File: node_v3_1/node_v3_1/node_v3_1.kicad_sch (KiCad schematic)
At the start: 69 parts, among them J1 Conn_Coaxial, J2 12402012E212A, J3 Micro_SD_Card, J4 VIN, J5 BAT, J7 DBG, J8 Conn_01x16_Pin, Q1 2N3904, U1 RST, U2 W25Q128JVS, U3 ADP2108AUJ-3.3, U4 RP2040, U5 RFM69HCW, U6 CAT3200-5, U7 MCP7940N-xSN, U8 MCP73831T-2ACI_OT, U9 BOOTSEL, Y1 445C35A12M00000, Y2 SC32S-7PF20PPM

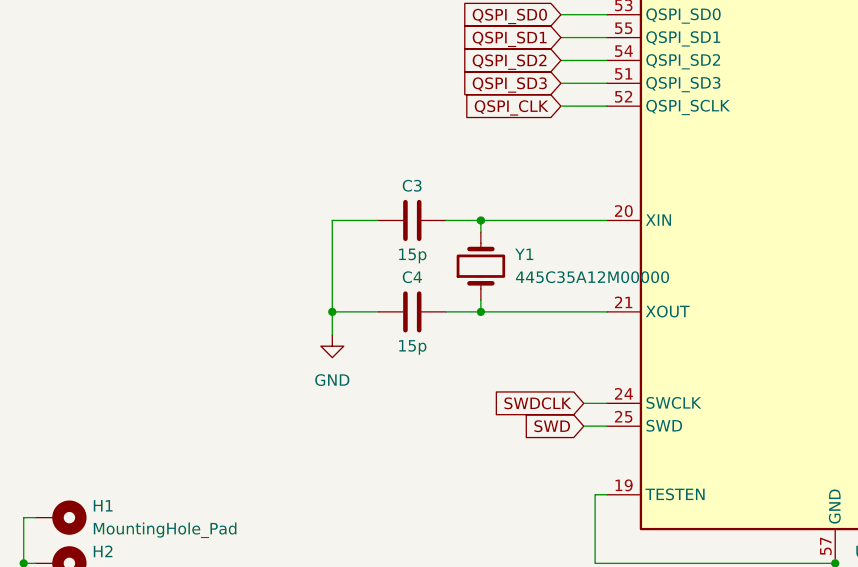
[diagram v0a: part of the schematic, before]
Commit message: updates
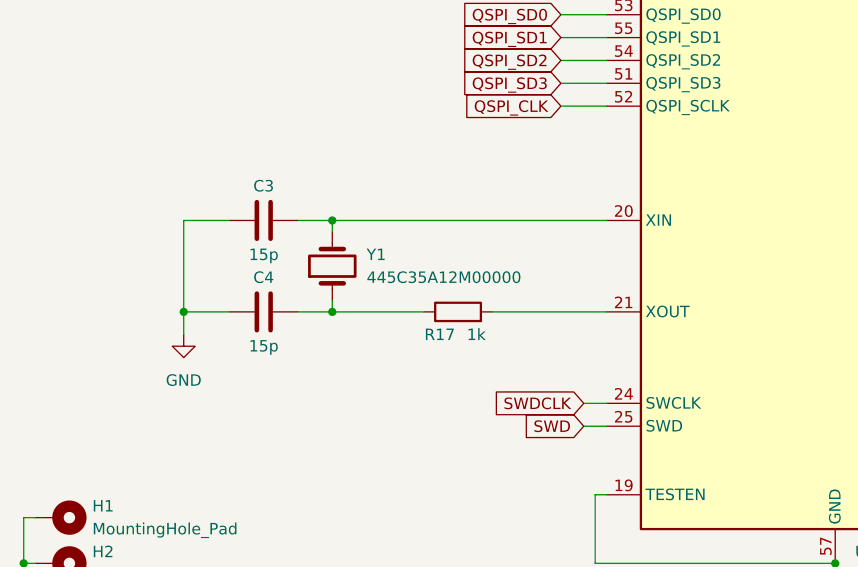
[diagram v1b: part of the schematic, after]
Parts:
- added R17: 1k, symbol Device:R
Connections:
- net at C4.2, Y1.1: now also R17.1; no longer U4.21 (XOUT)
- new net: R17.2, U4.21 (XOUT)
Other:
- moved on the sheet: C3, C4, Y1
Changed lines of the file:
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@@
 	)
 	(junction
-		(at 55.88 241.3)
+		(at 39.37 241.3)
 		(diameter 0)
 		(color 0 0 0 0)
@@
 	)
 	(junction
-		(at 72.39 241.3)
+		(at 55.88 231.14)
 		(diameter 0)
 		(color 0 0 0 0)
 	)
 	(junction
-		(at 72.39 231.14)
+		(at 250.19 248.92)
 		(diameter 0)
 		(color 0 0 0 0)
 	)
 	(junction
-		(at 250.19 248.92)
+		(at 46.99 123.19)
 		(diameter 0)
 		(color 0 0 0 0)
 	)
 	(junction
-		(at 46.99 123.19)
+		(at 21.59 279.4)
 		(diameter 0)
 		(color 0 0 0 0)
 	)
 	(junction
-		(at 21.59 279.4)
+		(at 55.88 241.3)
 		(diameter 0)
 		(color 0 0 0 0)
@@
 	(wire
 		(pts
-			(xy 72.39 240.03) (xy 72.39 241.3)
+			(xy 55.88 240.03) (xy 55.88 241.3)
 		)
 		(stroke
@@
 	(wire
 		(pts
-			(xy 72.39 232.41) (xy 72.39 231.14)
+			(xy 55.88 232.41) (xy 55.88 231.14)
 		)
 		(stroke
@@
 	(wire
 		(pts
-			(xy 72.39 231.14) (xy 86.36 231.14)
+			(xy 55.88 231.14) (xy 86.36 231.14)
 		)
 		(stroke
@@
 	(wire
 		(pts
+			(xy 73.66 241.3) (xy 86.36 241.3)
+		)
+		(stroke
+			(width 0)
+			(type default)
+		)
+	)
+	(wire
+		(pts
 			(xy 36.83 101.6) (xy 40.64 101.6)
 		)
@@
 	(wire
 		(pts
-			(xy 55.88 231.14) (xy 55.88 241.3)
+			(xy 39.37 231.14) (xy 39.37 241.3)
 		)
 		(stroke
@@
 	(wire
 		(pts
+			(xy 55.88 241.3) (xy 66.04 241.3)
+		)
+		(stroke
+			(width 0)
+			(type default)
+		)
+	)
+	(wire
+		(pts
 			(xy 246.38 226.06) (xy 246.38 229.87)
 		)
@@
 	(wire
 		(pts
-			(xy 60.96 231.14) (xy 55.88 231.14)
+			(xy 44.45 231.14) (xy 39.37 231.14)
 		)
 		(stroke
@@
 	(wire
 		(pts
-			(xy 55.88 241.3) (xy 60.96 241.3)
+			(xy 39.37 241.3) (xy 44.45 241.3)
 		)
 		(stroke
@@
 	(wire
 		(pts
-			(xy 55.88 241.3) (xy 55.88 243.84)
+			(xy 39.37 241.3) (xy 39.37 243.84)
 		)
 		(stroke
@@
 	(wire
 		(pts
-			(xy 72.39 241.3) (xy 86.36 241.3)
-		)
-		(stroke
-			(width 0)
-			(type default)
-		)
-	)
-	(wire
-		(pts
 			(xy 137.16 198.12) (xy 139.7 198.12)
 		)
@@
 	(wire
 		(pts
-			(xy 72.39 241.3) (xy 68.58 241.3)
+			(xy 55.88 241.3) (xy 52.07 241.3)
 		)
 		(stroke
@@
 	(wire
 		(pts
-			(xy 72.39 231.14) (xy 68.58 231.14)
+			(xy 55.88 231.14) (xy 52.07 231.14)
 		)
 		(stroke
@@
 	(symbol
 		(lib_id "Device:Crystal")
-		(at 72.39 236.22 90)
+		(at 55.88 236.22 90)
 		(unit 1)
 		(exclude_from_sim no)
@@
 		(on_board yes)
 		(dnp no)
-		(fields_autoplaced yes)
 		(property "Reference" "Y1"
-			(at 76.2 234.95 90)
+			(at 59.69 234.95 90)
 			(effects
 				(font
@@
 		)
 		(property "Value" "445C35A12M00000"
-			(at 76.2 237.49 90)
+			(at 59.69 237.49 90)
 			(effects
 				(font
@@
 		)
 		(property "Footprint" "custom:XTAL-445"
-			(at 72.39 236.22 0)
+			(at 55.88 236.22 0)
 			(effects
 				(font
@@
 		)
 		(property "Datasheet" "~"
-			(at 72.39 236.22 0)
+			(at 55.88 236.22 0)
 			(effects
 				(font
@@
 		)
 		(property "Description" ""
-			(at 72.39 236.22 0)
+			(at 55.88 236.22 0)
 			(effects
 				(font
@@
 		(lib_name "GND_2")
 		(lib_id "power:GND")
-		(at 55.88 243.84 0)
+		(at 39.37 243.84 0)
 		(unit 1)
 		(exclude_from_sim no)
@@
 		(fields_autoplaced yes)
 		(property "Reference" "#PWR023"
-			(at 55.88 250.19 0)
+			(at 39.37 250.19 0)
 			(effects
 				(font
@@
 		)
 		(property "Value" "GND"
-			(at 55.88 248.92 0)
+			(at 39.37 248.92 0)
 			(effects
 				(font
@@
 		)
 		(property "Footprint" ""
-			(at 55.88 243.84 0)
+			(at 39.37 243.84 0)
 			(effects
 				(font
@@
 		)
 		(property "Datasheet" ""
-			(at 55.88 243.84 0)
+			(at 39.37 243.84 0)
 			(effects
 				(font
@@
 		)
 		(property "Description" "Power symbol creates a global label with name \"GND\" , ground"
-			(at 55.88 243.84 0)
+			(at 39.37 243.84 0)
 			(effects
 				(font
@@
 	(symbol
 		(lib_id "Device:C")
-		(at 64.77 231.14 90)
+		(at 48.26 231.14 90)
 		(unit 1)
 		(exclude_from_sim no)
@@
 		(dnp no)
 		(property "Reference" "C3"
-			(at 64.77 227.33 90)
+			(at 48.26 227.33 90)
 			(effects
 				(font
@@
 		)
 		(property "Value" "15p"
-			(at 64.77 234.95 90)
+			(at 48.26 234.95 90)
 			(effects
 				(font
@@
 		)
 		(property "Footprint" "Capacitor_SMD:C_0402_1005Metric_Pad0.74x0.62mm_HandSolder"
-			(at 68.58 230.1748 0)
+			(at 52.07 230.1748 0)
 			(effects
 				(font
@@
 		)
 		(property "Datasheet" "~"
-			(at 64.77 231.14 0)
+			(at 48.26 231.14 0)
 			(effects
 				(font
@@
 		)
 		(property "Description" ""
-			(at 64.77 231.14 0)
+			(at 48.26 231.14 0)
 			(effects
 				(font
@@
 	)
 	(symbol
+		(lib_id "Device:R")
+		(at 69.85 241.3 90)
+		(unit 1)
+		(exclude_from_sim no)
+		(in_bom yes)
+		(on_board yes)
+		(dnp no)
+		(property "Reference" "R17"
+			(at 67.818 243.84 90)
+			(effects
+				(font
+					(size 1.27 1.27)
+				)
+			)
+		)
+		(property "Value" "1k"
+			(at 71.882 243.84 90)
+			(effects
+				(font
+					(size 1.27 1.27)
+				)
+			)
+		)
+		(property "Footprint" ""
+			(at 69.85 243.078 90)
+			(effects
+				(font
+					(size 1.27 1.27)
+				)
+				(hide yes)
+			)
+		)
+		(property "Datasheet" "~"
+			(at 69.85 241.3 0)
+			(effects
+				(font
+					(size 1.27 1.27)
+				)
+				(hide yes)
+			)
+		)
+		(property "Description" "Resistor"
+			(at 69.85 241.3 0)
+			(effects
+				(font
+					(size 1.27 1.27)
+				)
+				(hide yes)
+			)
+		)
+		(pin "2"
+		)
+		(pin "1"
+		)
+		(instances
+			(project ""
+				(path "/e774f05c-3d76-4c30-8e02-47afd946aaf5"
+					(reference "R17")
+					(unit 1)
+				)
+			)
+		)
+	)
+	(symbol
 		(lib_name "GND_2")
 		(lib_id "power:GND")
@@
 	(symbol
 		(lib_id "Device:C")
-		(at 64.77 241.3 90)
+		(at 48.26 241.3 90)
 		(unit 1)
 		(exclude_from_sim no)
@@
 		(dnp no)
 		(property "Reference" "C4"
-			(at 64.77 237.49 90)
+			(at 48.26 237.49 90)
 			(effects
 				(font
@@
 		)
 		(property "Value" "15p"
-			(at 64.77 245.11 90)
+			(at 48.26 245.11 90)
 			(effects
 				(font
@@
 		)
 		(property "Footprint" "Capacitor_SMD:C_0402_1005Metric_Pad0.74x0.62mm_HandSolder"
-			(at 68.58 240.3348 0)
+			(at 52.07 240.3348 0)
 			(effects
 				(font
@@
 		)
 		(property "Datasheet" "~"
-			(at 64.77 241.3 0)
+			(at 48.26 241.3 0)
 			(effects
 				(font
@@
 		)
 		(property "Description" ""
-			(at 64.77 241.3 0)
+			(at 48.26 241.3 0)
 			(effects
 				(font
